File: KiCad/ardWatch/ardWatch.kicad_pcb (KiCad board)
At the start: 2 copper layers, 66 x 58.4 mm, 4 parts, among them J1 2-pin_power_input_header, U1 Arduino_Mini_Pro, U3 ST7735_1.8"_TFT_128x160, U4 DS3231_RTC_module

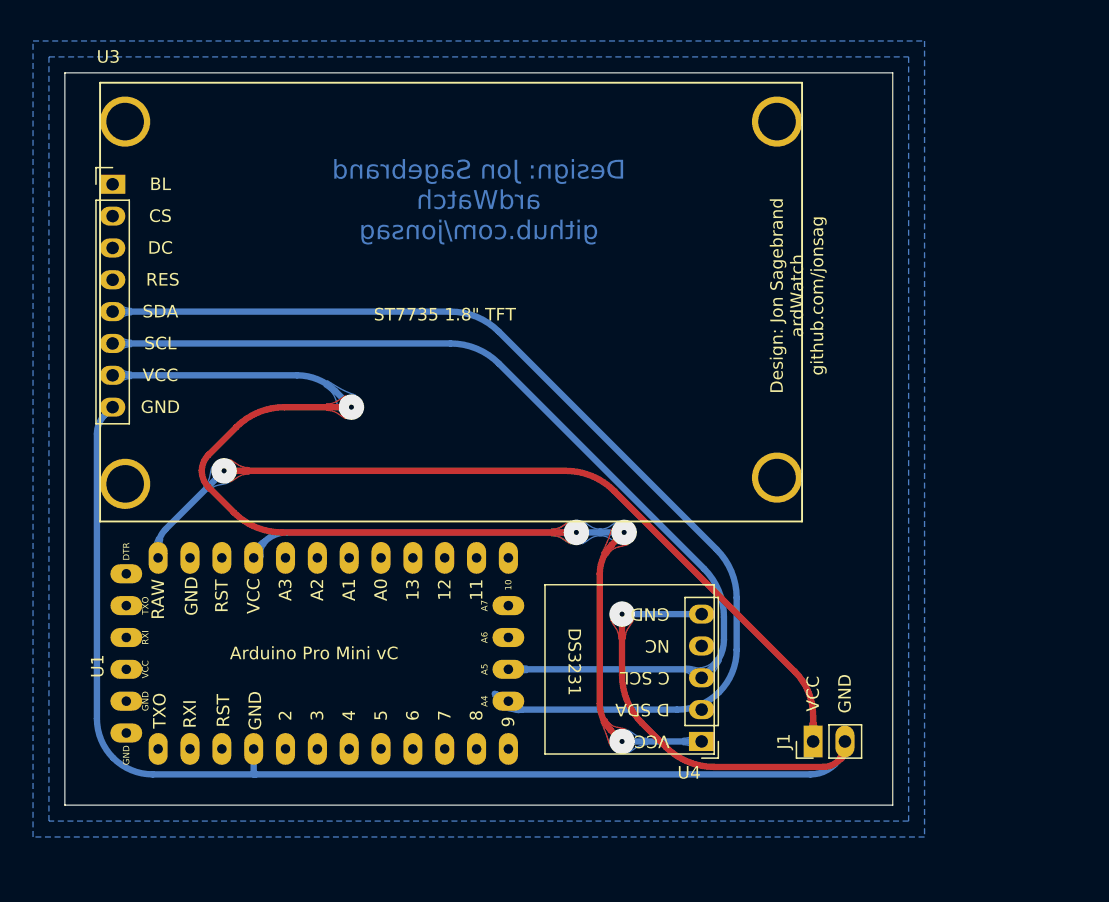
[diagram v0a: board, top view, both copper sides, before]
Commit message: pcb
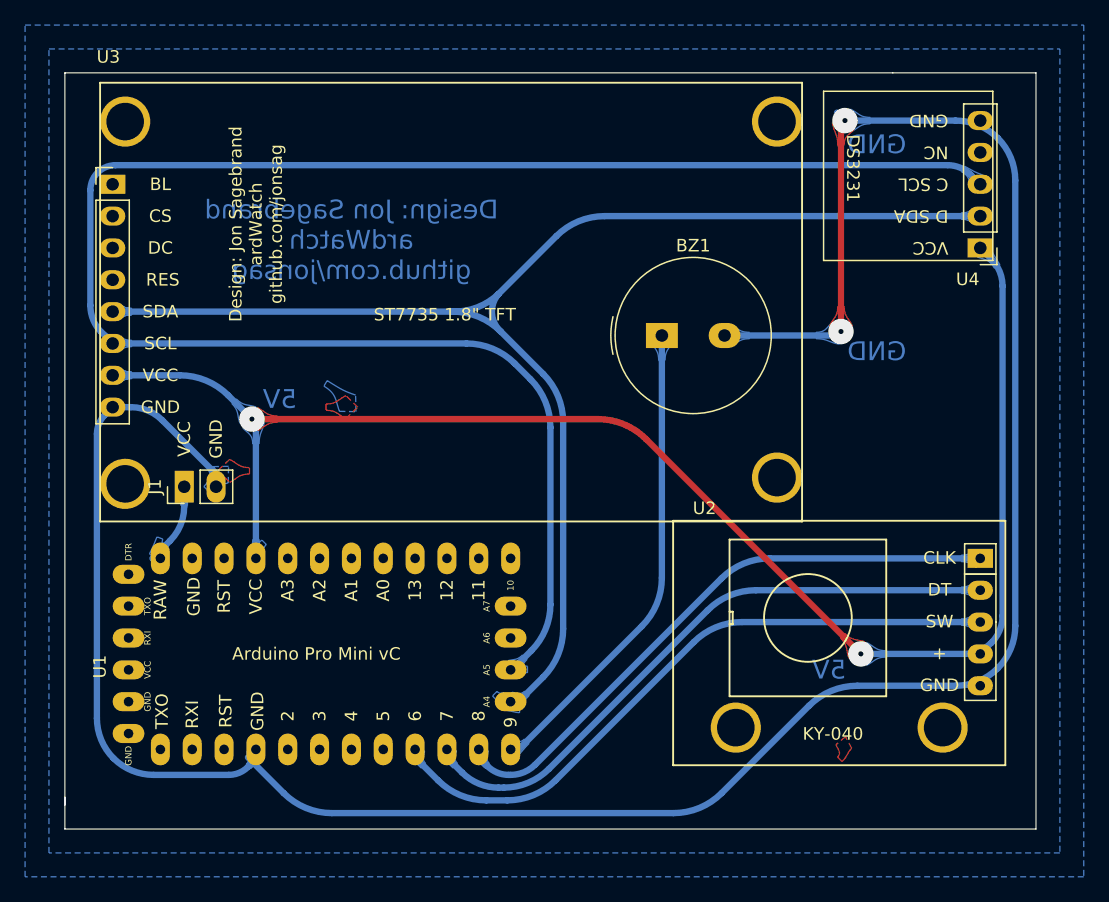
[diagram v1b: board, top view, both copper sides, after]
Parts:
- added BZ1: Buzzer, My_Misc:Buzzer_TDK_PS1240P02BT_D12.2mm_H6.5mm_large, F.Cu at (123.8, 70.5)
- added U2: KY-040_Rotary_Encoder, My_Parts:KY-040_rotary_encoder module_w_header_large, F.Cu at (149.2, 88.3)
- moved J1 54.1 mm to (85.7, 82.5)
- moved U4 45.2 mm to (149.2, 63.5)
- moved U1 4.29 mm to (83.8, 103.5)
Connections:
- U1 pad 10: unconnected-(U1-Pad10) -> Net-(U2-Pad2)
- U1 pad 11: unconnected-(U1-Pad11) -> Net-(U2-Pad1)
- U1 pad 12: unconnected-(U1-Pad12) -> Net-(U1-Pad12)
- U1 pad 9: unconnected-(U1-Pad9) -> Net-(U2-Pad3)
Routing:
- net GND: track 125.2 -> 201.4 mm, vias 1 -> 2
- net SCL: track 79.5 -> 144.2 mm
- net VCC: track 66.9 -> 6.58 mm, vias 1 -> 0
- net Net-(U2-Pad3): track 0.00 -> 52.2 mm
- net Net-(U2-Pad2): track 0.00 -> 50.0 mm
- net Net-(U2-Pad1): track 0.00 -> 47.8 mm
- net Net-(U1-Pad12): track 0.00 -> 37.5 mm
- net SDA: track 86.6 -> 112.5 mm
- net +5V: track 120.2 -> 122.5 mm, vias 4 -> 2
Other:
- board size 66 x 58.4 mm -> 77.5 x 60.3 mm
- board text added: "5V"
- board text added: "GND"
